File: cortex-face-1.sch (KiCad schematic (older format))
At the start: 170 parts, among them J1 Conn_01x04, SW1 SW_Push, U1 Elite-C

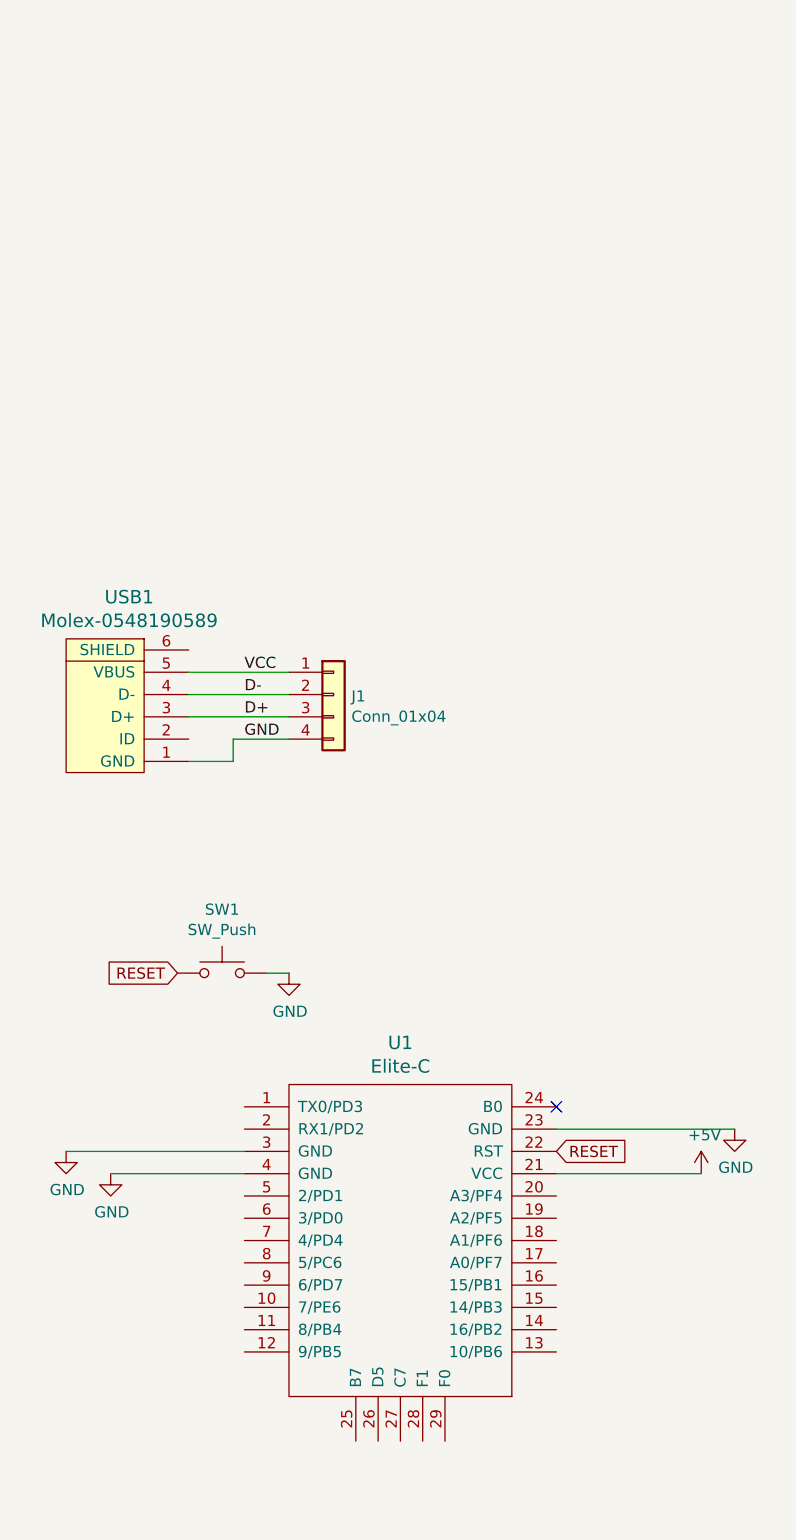
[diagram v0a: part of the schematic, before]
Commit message: First pass at routing
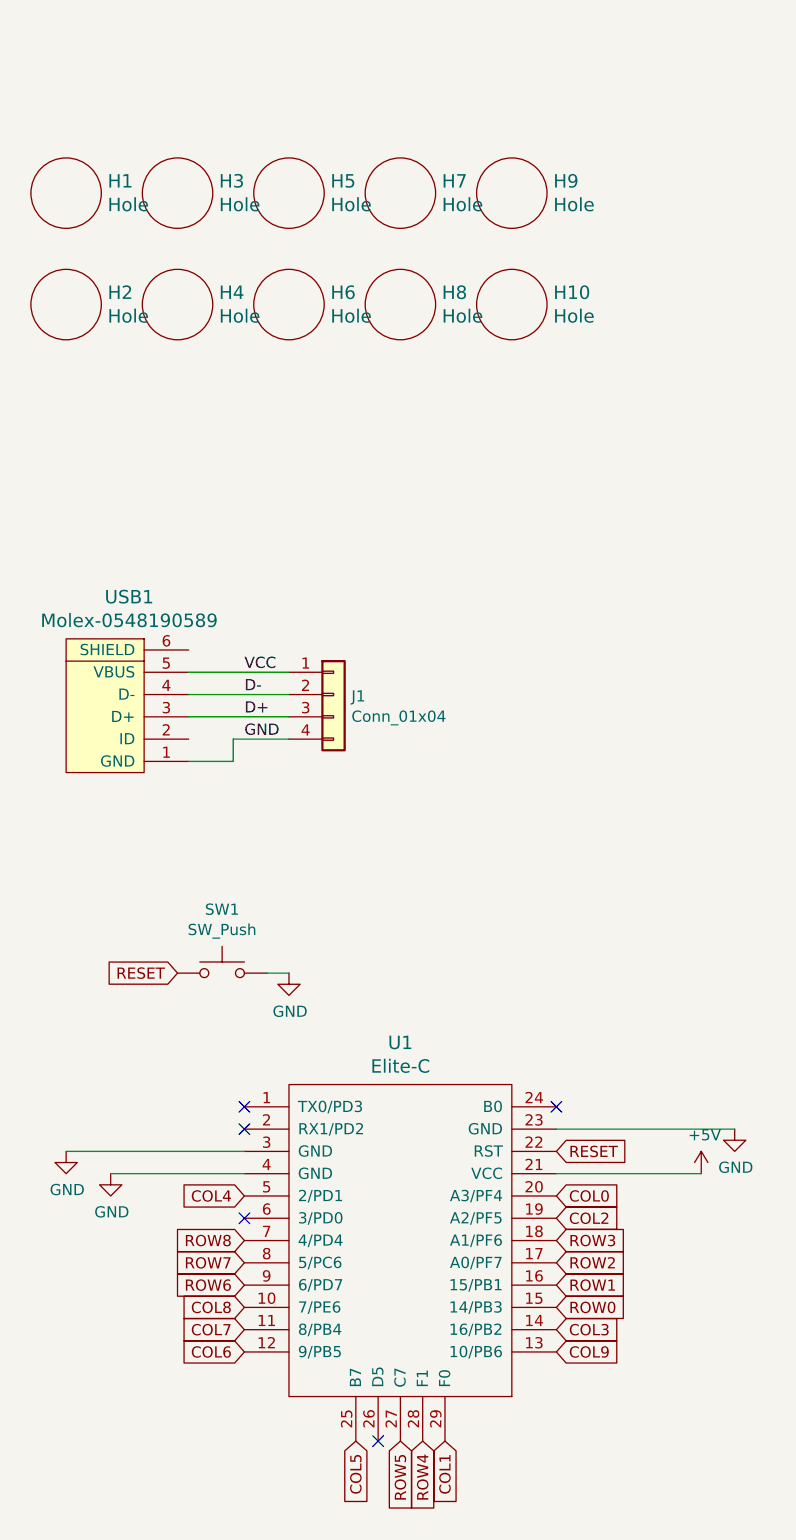
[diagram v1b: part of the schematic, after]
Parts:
- added H1, H10, H2, H3, H4, H5, H6, H7, H8, H9: Hole, MountingHole:MountingHole_6mm, symbol keebio:Hole
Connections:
- net COL0: now also U1.20 (A3/PF4)
- net COL1: now also U1.29 (F0)
- net COL2: now also U1.19 (A2/PF5)
- net COL3: now also U1.14 (16/PB2)
- net COL4: now also U1.5 (2/PD1)
- net COL5: now also U1.25 (B7)
- net COL6: now also U1.12 (9/PB5)
- net COL7: now also U1.11 (8/PB4)
- net COL8: now also U1.10 (7/PE6)
- net COL9: now also U1.13 (10/PB6)
- net ROW0: now also U1.15 (14/PB3)
- net ROW1: now also U1.16 (15/PB1)
- net ROW2: now also U1.17 (A0/PF7)
- net ROW3: now also U1.18 (A1/PF6)
- net ROW4: now also U1.28 (F1)
- net ROW5: now also U1.27 (C7)
- net ROW6: now also U1.9 (6/PD7)
- net ROW7: now also U1.8 (5/PC6)
- net ROW8: now also U1.7 (4/PD4)
- no-connect marks 1 -> 5
